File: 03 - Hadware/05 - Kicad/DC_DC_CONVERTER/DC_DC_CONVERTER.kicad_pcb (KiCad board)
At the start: 2 copper layers, 87 parts, among them J2 USB_B, J3 Screw_Terminal_01x02, J4 Screw_Terminal_01x02, K1 SRD-05VDC-SL-C, K2 SRD-05VDC-SL-C, K3 SRD-05VDC-SL-C, K4 SRD-05VDC-SL-C, Q1 BC547, Q10 IRLZ44N, Q2 IRLZ44N, Q27 IRLZ44N, Q28 IRLZ44N, Q3 BC547, Q32 IRLZ44N, Q33 IRLZ44N, Q34 IRLZ44N, Q35 IRLZ44N, Q36 IRLZ44N, Q4 IRLZ44N, Q5 BC547, Q6 IRLZ44N, Q7 BC547, U2 LT1083-ADJ, U3 ATmega328P-P, U4 CH340G, U5 LCD-16X2, U6 LM2576HVT-5.0, U8 IR2104, U9 IR2104, Y1 16MHz, Y2 12MHz

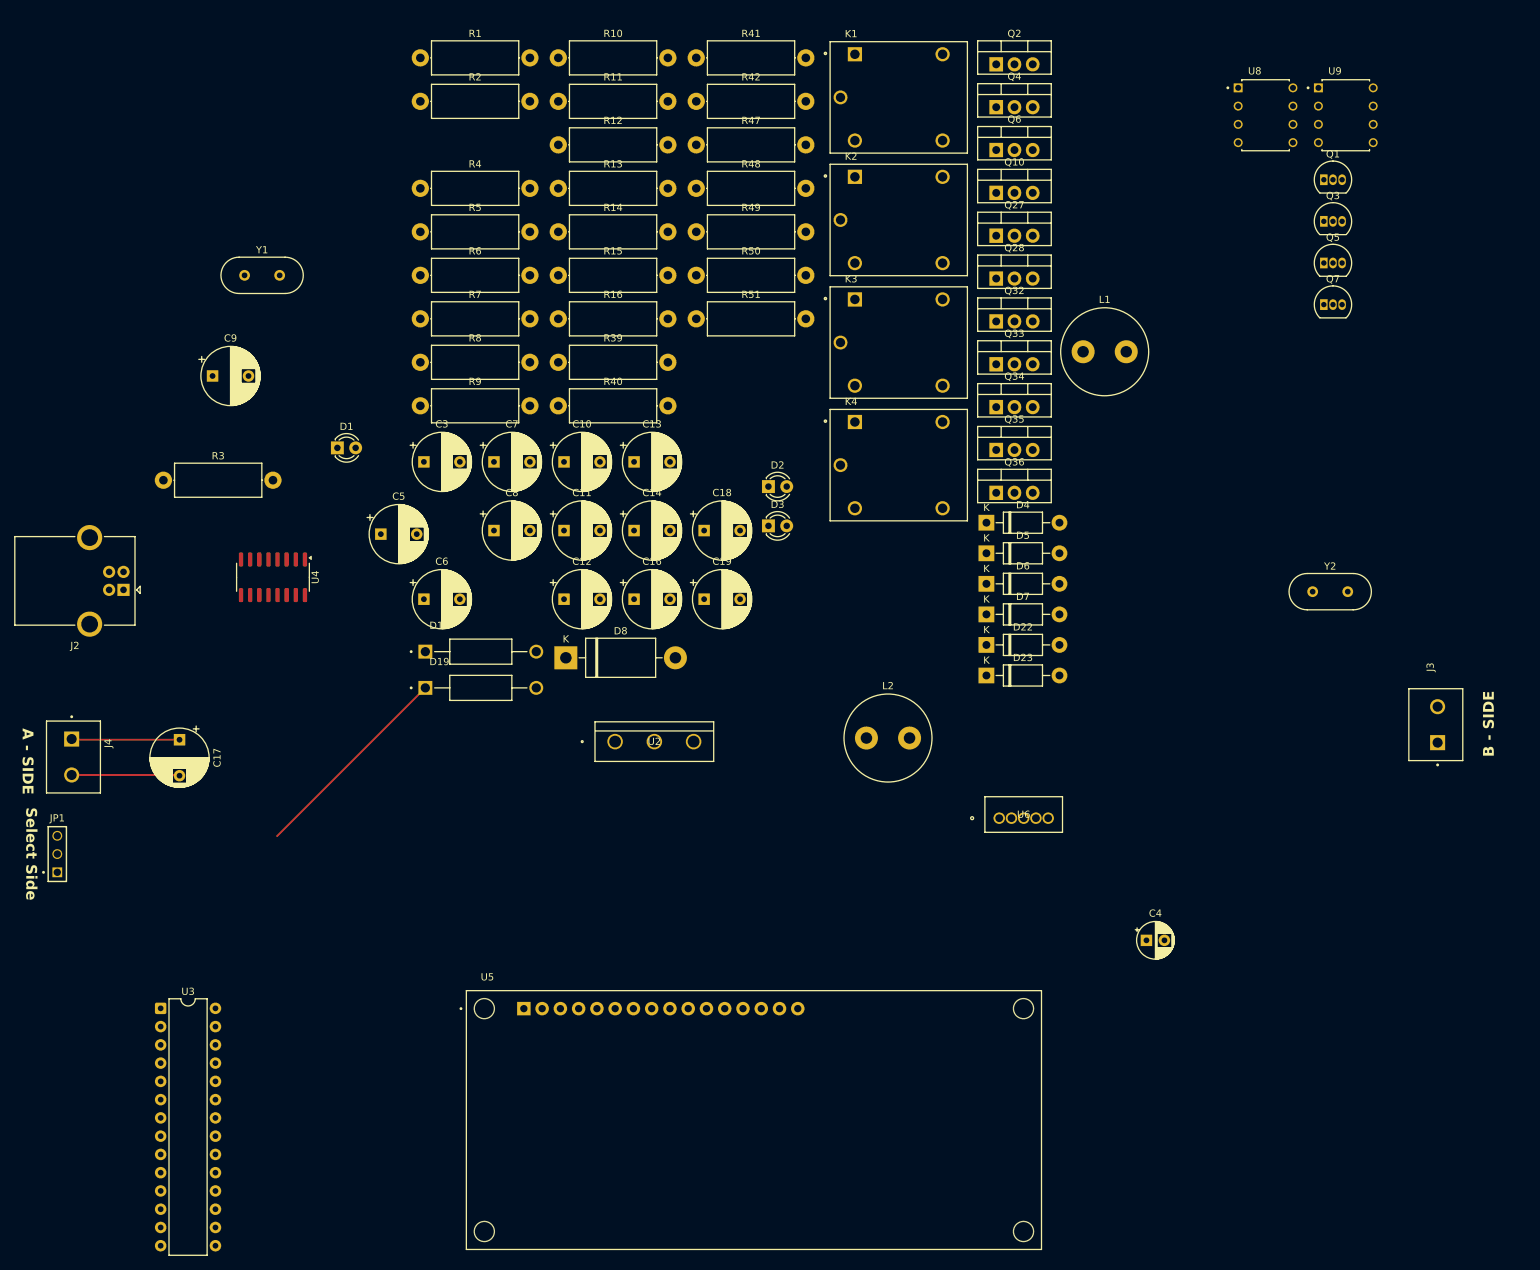
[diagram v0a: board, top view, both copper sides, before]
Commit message: release pires 18.05.25 update: Schematic/Layout/Priteus simulation/Matlab Simulation/Monogroph
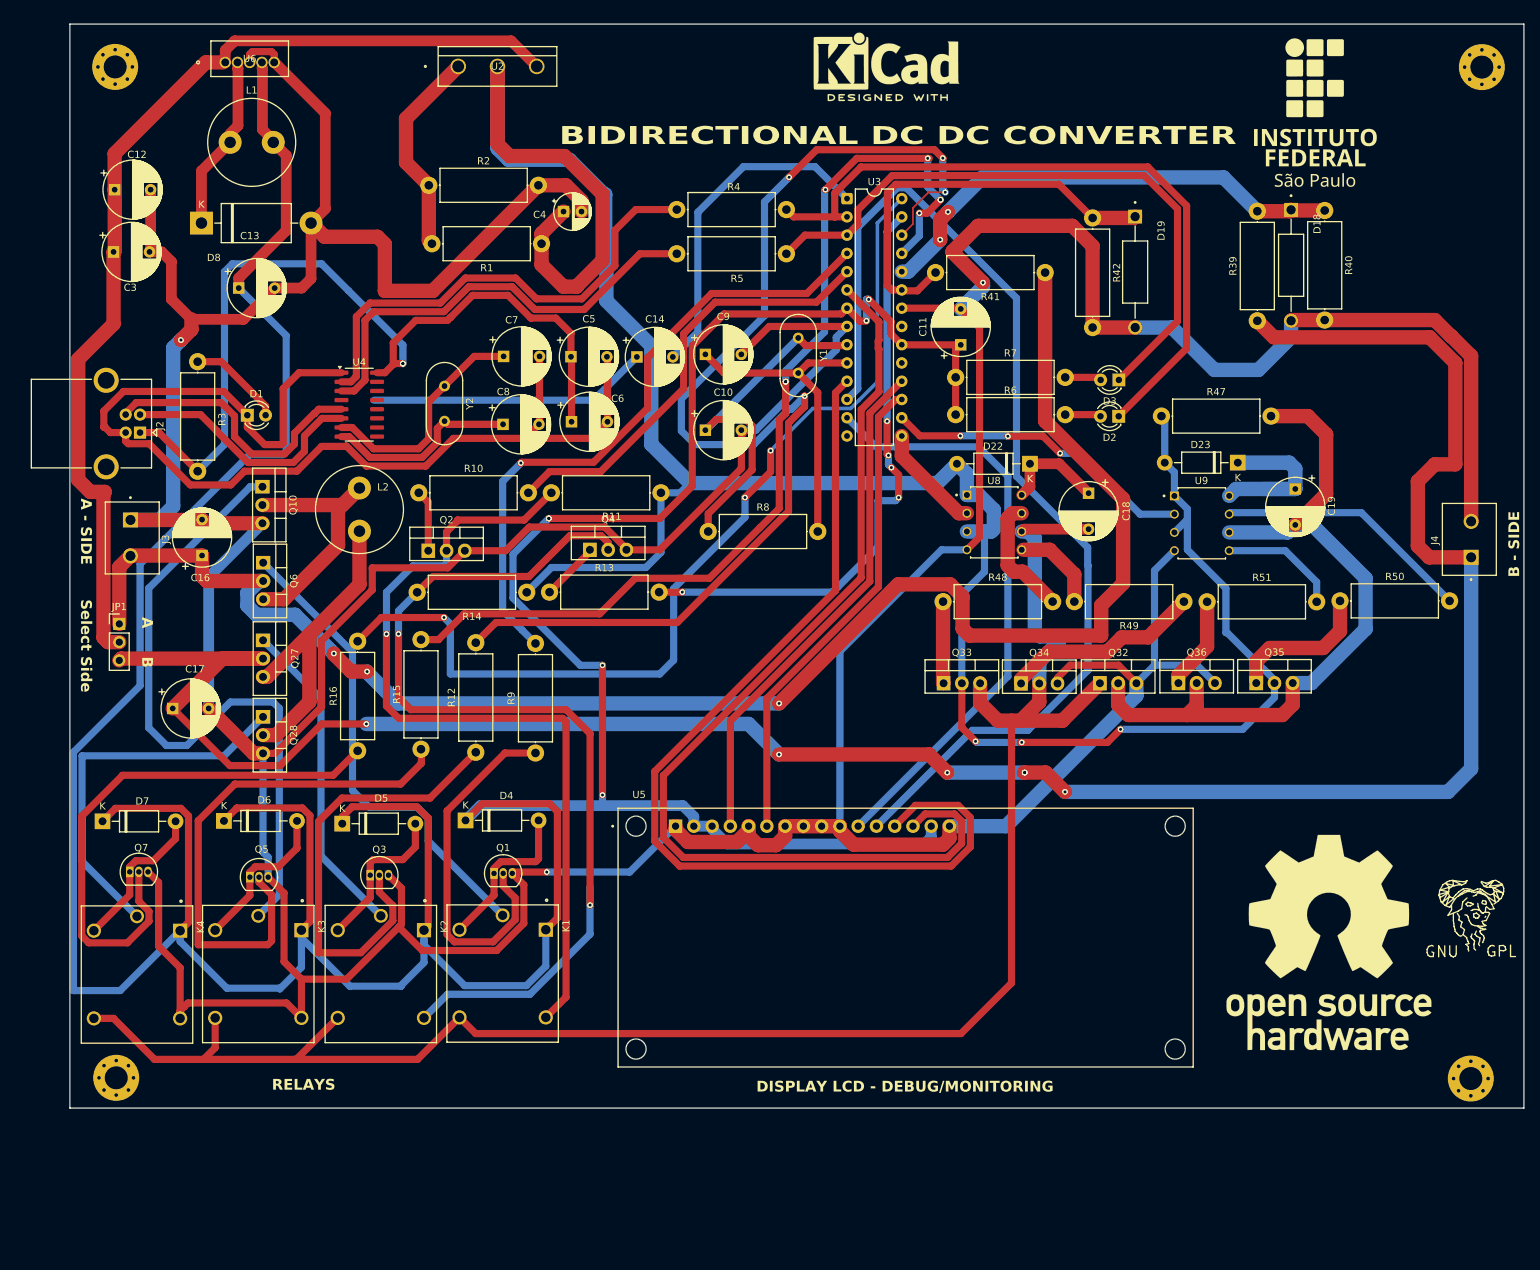
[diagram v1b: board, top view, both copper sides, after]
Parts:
- added G***: LOGO, Logo:Logo_IFSP, F.Cu at (211.0, 26.4)
- added REF**: MountingHole_3.2mm_M3_Pad_Via, MountingHole:MountingHole_3.2mm_M3_Pad_Via, F.Cu at (232.6, 160.7)
- added REF**: Symbol_GNU-Logo_SilkscreenTop, Symbol:Symbol_GNU-Logo_SilkscreenTop, F.Cu at (232.9, 136.9)
- added REF**: MountingHole_3.2mm_M3_Pad_Via, MountingHole:MountingHole_3.2mm_M3_Pad_Via, F.Cu at (234.2, 20.0)
- added REF**: KiCad-Logo2_8mm_SilkScreen, Symbol:KiCad-Logo2_8mm_SilkScreen, F.Cu at (151.3, 19.2)
- added REF**: OSHW-Logo_28.5x30mm_SilkScreen, Symbol:OSHW-Logo_28.5x30mm_SilkScreen, F.Cu at (212.9, 141.8)
- added REF**: MountingHole_3.2mm_M3_Pad_Via, MountingHole:MountingHole_3.2mm_M3_Pad_Via, F.Cu at (44.2, 160.6)
- added REF**: MountingHole_3.2mm_M3_Pad_Via, MountingHole:MountingHole_3.2mm_M3_Pad_Via, F.Cu at (44.0, 20.0)
- JP1: footprint Library:SAMTEC_MTSW-101-06-T-T-100 -> Connector_PinHeader_2.54mm:PinHeader_1x03_P2.54mm_Vertical
- moved J4 197.0 mm to (232.7, 85.7), turned to 90 degrees
- moved Q7 183.9 mm to (46.1, 132.0)
- moved J3 183.7 mm to (46.2, 85.5), turned to -90 degrees
- moved Q5 172.1 mm to (62.8, 132.7)
- moved Q3 160.8 mm to (79.5, 132.4)
- moved U6 150.5 mm to (59.4, 19.4)
- moved Q1 150.4 mm to (96.7, 132.2)
- moved U3 147.6 mm to (145.8, 38.3)
- moved K1 133.7 mm to (97.9, 146.1), turned to -90 degrees
- moved C4 129.8 mm to (106.4, 40.1)
- moved K4 127.5 mm to (47.1, 146.3), turned to -90 degrees
- moved K2 127.2 mm to (81.0, 146.2), turned to -90 degrees
- moved D7 126.3 mm to (42.3, 124.9)
- moved K3 125.1 mm to (64.0, 146.2), turned to -90 degrees
- moved D18 124.9 mm to (207.6, 47.6), turned to -90 degrees
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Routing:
- net GND: track 15.0 -> 867.5 mm, vias 0 -> 3
- net 5V: track 0.00 -> 587.4 mm, vias 0 -> 6
- net 17V: track 0.00 -> 343.9 mm, vias 0 -> 3
- net B_Side: track 15.0 -> 323.9 mm, vias 0 -> 6
- net D: track 0.00 -> 252.1 mm
- net A_Side: track 0.00 -> 230.3 mm, vias 0 -> 3
- net Control_R3A: track 0.00 -> 168.7 mm, vias 0 -> 4
- net GND1: track 0.00 -> 150.4 mm
- net D5: track 0.00 -> 149.6 mm
- net D7: track 0.00 -> 145.0 mm
- net POWER: track 0.00 -> 142.0 mm
- net D6: track 0.00 -> 138.0 mm
- net Control_R2A: track 0.00 -> 137.5 mm, vias 0 -> 7
- net Net-(Q4-D): track 0.00 -> 134.1 mm, vias 0 -> 2
- net Control_R4A: track 0.00 -> 134.0 mm, vias 0 -> 3
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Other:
- board outline added: 202.3 x 150.8 mm
- board text added: "A"
- board text added: "B"
- board text added: "BIDIRECTIONAL DC DC CONVERTER"
- board text added: "DISPLAY LCD - DEBUG/MONITORING"
- board text added: "RELAYS"

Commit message: add picture folder
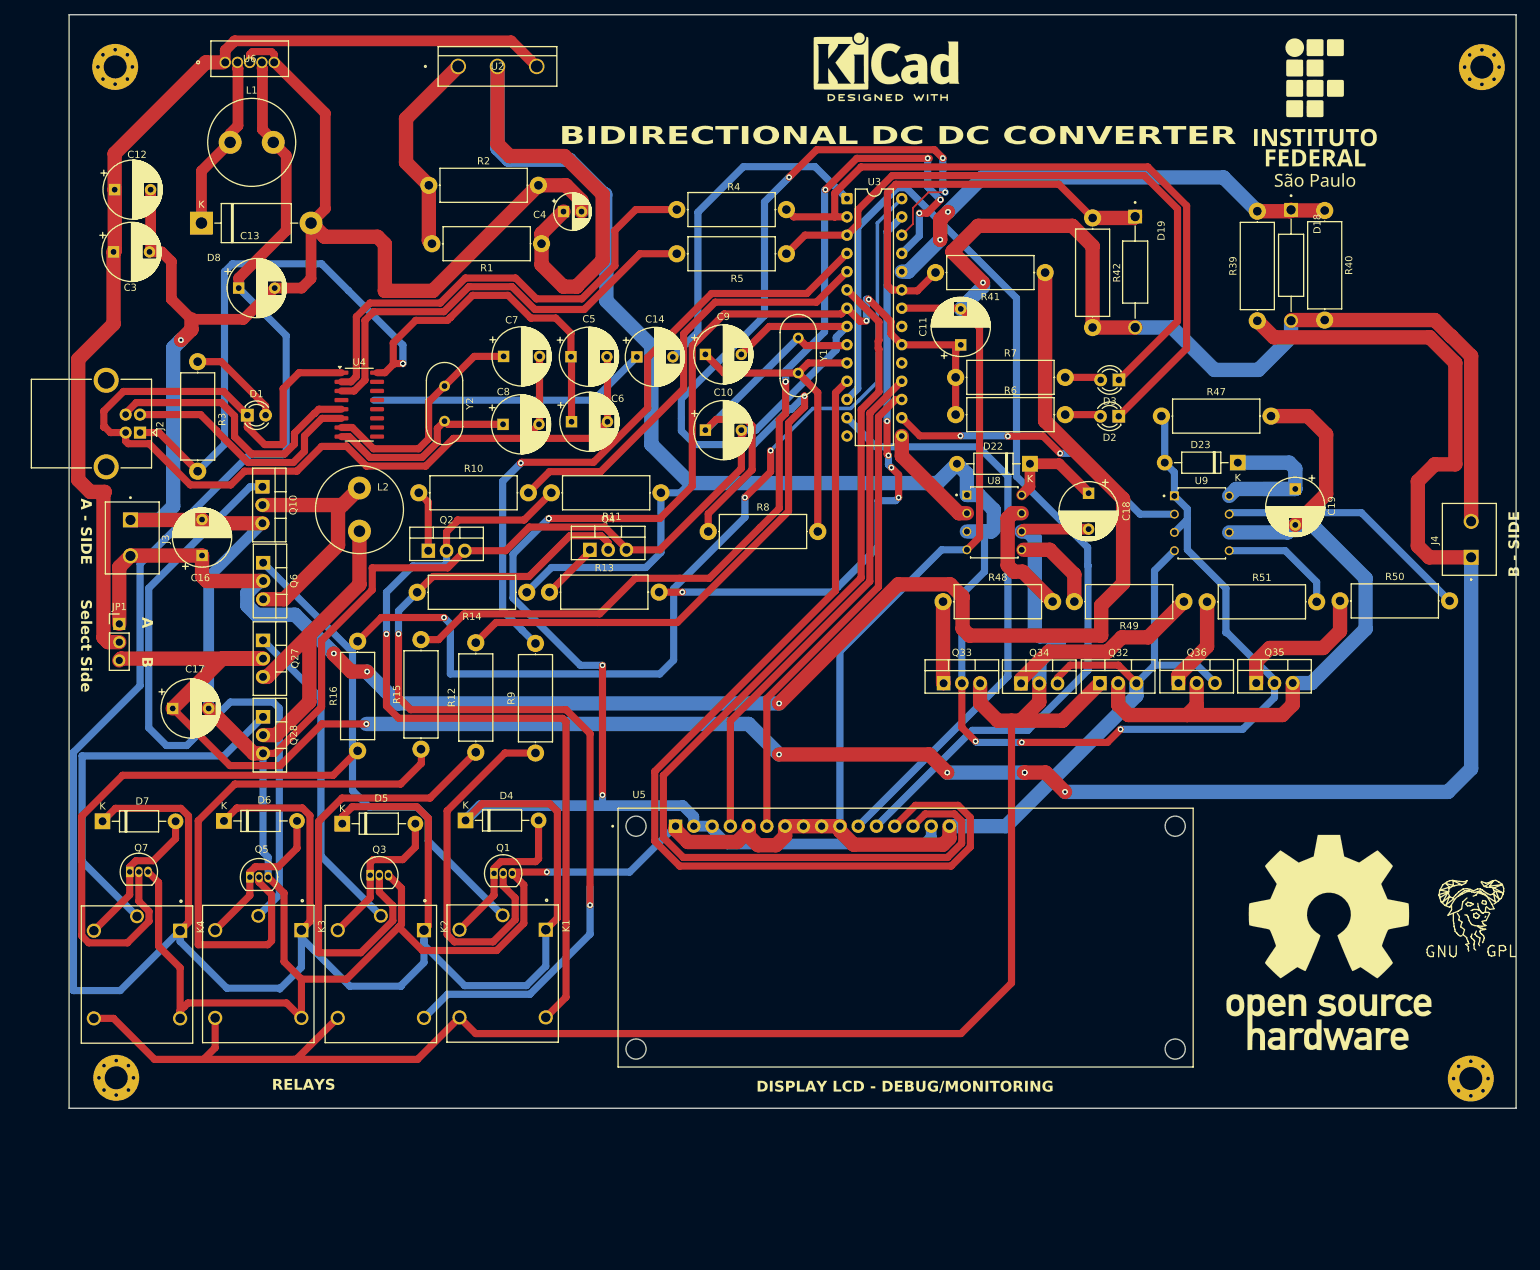
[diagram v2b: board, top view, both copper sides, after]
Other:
- board size 202.3 x 150.8 mm -> 201.3 x 152.1 mm
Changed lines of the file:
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@@
 	)
 	(gr_rect
-		(start 37.7444 14.0462)
-		(end 240.0046 164.8333)
+		(start 37.6428 12.7508)
+		(end 238.9124 164.8587)
 		(stroke
 			(width 0.1)
